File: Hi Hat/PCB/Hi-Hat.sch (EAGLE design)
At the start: 91 parts, among them IC1 LM741P, IC2 LM741P, IC3 LM741P, IC4 LM741P, IC5 LM741P, IC6 LM741P, IC7 LM741P, Q1 2N2222A, Q6 2N3904, Q7 2N3904

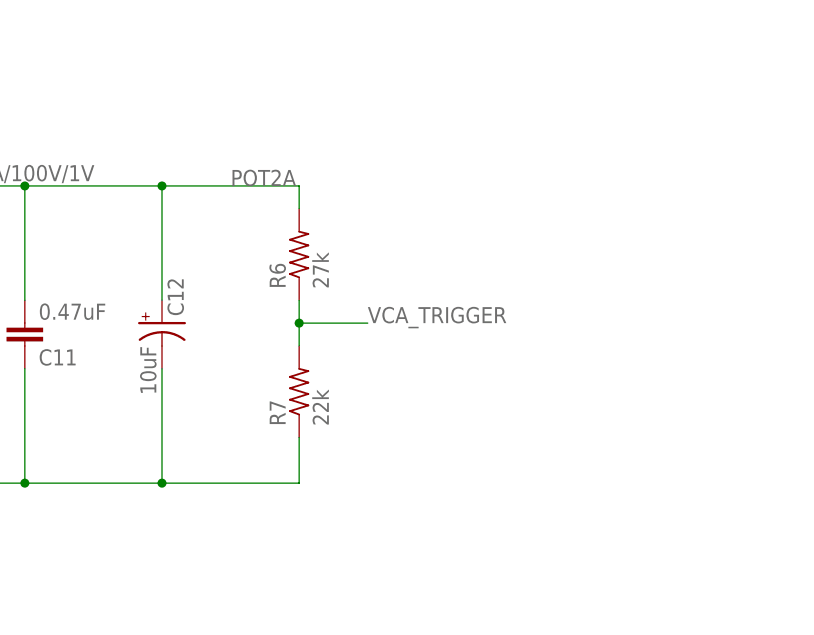
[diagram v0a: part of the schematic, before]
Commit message: Worked more on cymbals
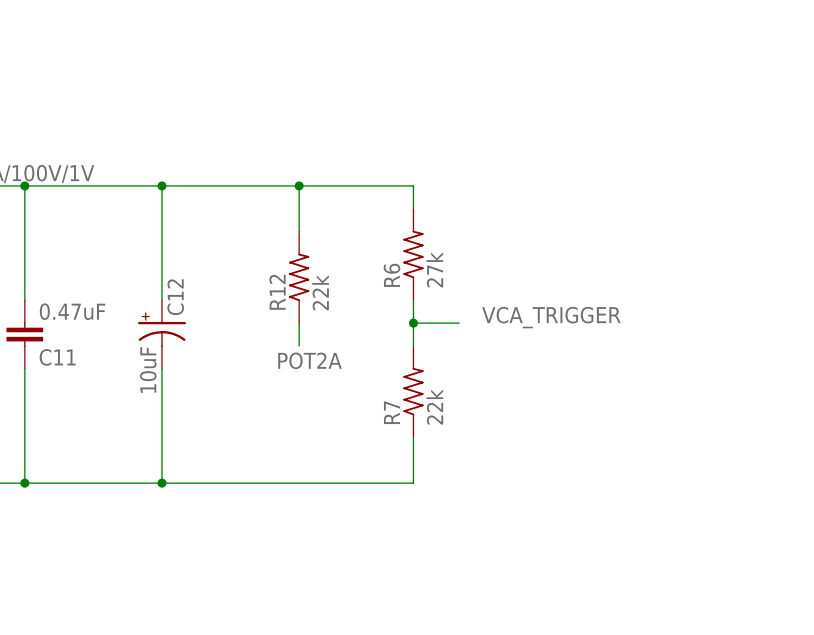
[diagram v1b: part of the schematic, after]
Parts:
- added R12: 22k, rcl:R-US_0207/7
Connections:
- new net N$6: C11.2, C12.+, D1.C, R12.2, R6.2
- net POT2A: now also R12.1; no longer C11.2, C12.+, D1.C, R6.2
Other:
- moved on the sheet: R6, R7
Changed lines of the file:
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@@
 <part name="TRIM1" library="Capstone" deviceset="10K_TRIMMER" device="" value="10k"/>
 <part name="TRIM2" library="Capstone" deviceset="10K_TRIMMER" device="" value="10k"/>
+<part name="R12" library="rcl" library_urn="urn:adsk.eagle:library:334" deviceset="R-US_" device="0207/7" package3d_urn="urn:adsk.eagle:package:23493/1" value="22k"/>
 </parts>
 <sheets>
@@
 <attribute name="VALUE" x="1661.922" y="334.01" size="1.778" layer="96" rot="R90"/>
 </instance>
-<instance part="R6" gate="G$1" x="693.42" y="358.14" smashed="yes" rot="R90">
-<attribute name="NAME" x="691.9214" y="354.33" size="1.778" layer="95" rot="R90"/>
-<attribute name="VALUE" x="696.722" y="354.33" size="1.778" layer="96" rot="R90"/>
-</instance>
-<instance part="R7" gate="G$1" x="693.42" y="342.9" smashed="yes" rot="R90">
-<attribute name="NAME" x="691.9214" y="339.09" size="1.778" layer="95" rot="R90"/>
-<attribute name="VALUE" x="696.722" y="339.09" size="1.778" layer="96" rot="R90"/>
+<instance part="R6" gate="G$1" x="706.12" y="358.14" smashed="yes" rot="R90">
+<attribute name="NAME" x="704.6214" y="354.33" size="1.778" layer="95" rot="R90"/>
+<attribute name="VALUE" x="709.422" y="354.33" size="1.778" layer="96" rot="R90"/>
+</instance>
+<instance part="R7" gate="G$1" x="706.12" y="342.9" smashed="yes" rot="R90">
+<attribute name="NAME" x="704.6214" y="339.09" size="1.778" layer="95" rot="R90"/>
+<attribute name="VALUE" x="709.422" y="339.09" size="1.778" layer="96" rot="R90"/>
 </instance>
 <instance part="R5" gate="G$1" x="640.08" y="347.98" smashed="yes" rot="R90">
@@
 <attribute name="NAME" x="1213.231" y="359.41" size="1.778" layer="95" rot="R90"/>
 <attribute name="VALUE" x="1215.39" y="359.41" size="1.778" layer="96" rot="R90"/>
+</instance>
+<instance part="R12" gate="G$1" x="693.42" y="355.6" smashed="yes" rot="R90">
+<attribute name="NAME" x="691.9214" y="351.79" size="1.778" layer="95" rot="R90"/>
+<attribute name="VALUE" x="696.722" y="351.79" size="1.778" layer="96" rot="R90"/>
 </instance>
 </instances>
@@
 </segment>
 <segment>
-<pinref part="D1" gate="G$1" pin="C"/>
-<wire x1="652.78" y1="365.76" x2="662.94" y2="365.76" width="0.1524" layer="91"/>
-<pinref part="R6" gate="G$1" pin="2"/>
-<wire x1="662.94" y1="365.76" x2="678.18" y2="365.76" width="0.1524" layer="91"/>
-<wire x1="678.18" y1="365.76" x2="693.42" y2="365.76" width="0.1524" layer="91"/>
-<wire x1="693.42" y1="365.76" x2="693.42" y2="363.22" width="0.1524" layer="91"/>
-<pinref part="C11" gate="G$1" pin="2"/>
-<wire x1="662.94" y1="353.06" x2="662.94" y2="365.76" width="0.1524" layer="91"/>
-<junction x="662.94" y="365.76"/>
-<pinref part="C12" gate="G$1" pin="+"/>
-<wire x1="678.18" y1="353.06" x2="678.18" y2="365.76" width="0.1524" layer="91"/>
-<junction x="678.18" y="365.76"/>
-<label x="685.8" y="365.76" size="1.778" layer="95"/>
+<pinref part="R12" gate="G$1" pin="1"/>
+<wire x1="693.42" y1="350.52" x2="693.42" y2="347.98" width="0.1524" layer="91"/>
+<label x="690.88" y="345.44" size="1.778" layer="95"/>
 </segment>
 </net>
@@
 <wire x1="662.94" y1="332.74" x2="662.94" y2="345.44" width="0.1524" layer="91"/>
 <label x="657.86" y="330.2" size="1.778" layer="95" rot="MR0"/>
-<wire x1="693.42" y1="337.82" x2="693.42" y2="332.74" width="0.1524" layer="91"/>
-<wire x1="693.42" y1="332.74" x2="678.18" y2="332.74" width="0.1524" layer="91"/>
+<wire x1="706.12" y1="337.82" x2="706.12" y2="332.74" width="0.1524" layer="91"/>
+<wire x1="706.12" y1="332.74" x2="678.18" y2="332.74" width="0.1524" layer="91"/>
 <junction x="662.94" y="332.74"/>
 <pinref part="R7" gate="G$1" pin="1"/>
@@
 </segment>
 <segment>
-<wire x1="693.42" y1="353.06" x2="693.42" y2="350.52" width="0.1524" layer="91"/>
+<wire x1="706.12" y1="353.06" x2="706.12" y2="350.52" width="0.1524" layer="91"/>
 <pinref part="R6" gate="G$1" pin="1"/>
 <pinref part="R7" gate="G$1" pin="2"/>
-<wire x1="693.42" y1="350.52" x2="693.42" y2="347.98" width="0.1524" layer="91"/>
-<wire x1="693.42" y1="350.52" x2="701.04" y2="350.52" width="0.1524" layer="91"/>
-<junction x="693.42" y="350.52"/>
-<label x="701.04" y="350.52" size="1.778" layer="95"/>
+<wire x1="706.12" y1="350.52" x2="706.12" y2="347.98" width="0.1524" layer="91"/>
+<wire x1="706.12" y1="350.52" x2="711.2" y2="350.52" width="0.1524" layer="91"/>
+<junction x="706.12" y="350.52"/>
+<label x="713.74" y="350.52" size="1.778" layer="95"/>
 </segment>
 <segment>
@@
 </segment>
 </net>
+<net name="N$6" class="0">
+<segment>
+<pinref part="D1" gate="G$1" pin="C"/>
+<pinref part="R6" gate="G$1" pin="2"/>
+<wire x1="652.78" y1="365.76" x2="662.94" y2="365.76" width="0.1524" layer="91"/>
+<wire x1="662.94" y1="365.76" x2="678.18" y2="365.76" width="0.1524" layer="91"/>
+<wire x1="678.18" y1="365.76" x2="693.42" y2="365.76" width="0.1524" layer="91"/>
+<wire x1="693.42" y1="365.76" x2="706.12" y2="365.76" width="0.1524" layer="91"/>
+<wire x1="706.12" y1="365.76" x2="706.12" y2="363.22" width="0.1524" layer="91"/>
+<pinref part="R12" gate="G$1" pin="2"/>
+<wire x1="693.42" y1="360.68" x2="693.42" y2="365.76" width="0.1524" layer="91"/>
+<junction x="693.42" y="365.76"/>
+<pinref part="C12" gate="G$1" pin="+"/>
+<wire x1="678.18" y1="353.06" x2="678.18" y2="365.76" width="0.1524" layer="91"/>
+<junction x="678.18" y="365.76"/>
+<pinref part="C11" gate="G$1" pin="2"/>
+<wire x1="662.94" y1="353.06" x2="662.94" y2="365.76" width="0.1524" layer="91"/>
+<junction x="662.94" y="365.76"/>
+</segment>
+</net>
